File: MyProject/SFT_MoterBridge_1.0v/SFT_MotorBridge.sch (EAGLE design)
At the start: 44 parts

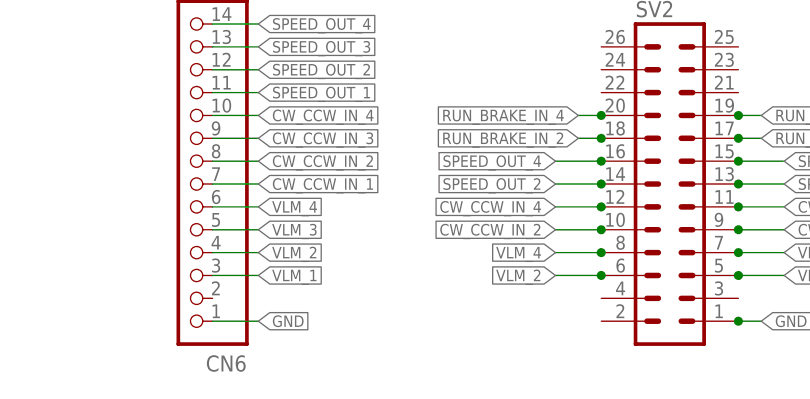
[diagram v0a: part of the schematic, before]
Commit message: kyuukei reset
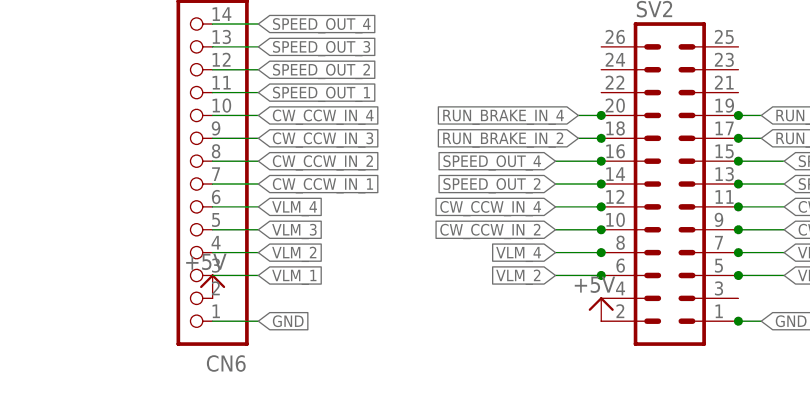
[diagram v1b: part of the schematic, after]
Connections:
- net +5V: now also CN6.2, SV2.2
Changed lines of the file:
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@@
 <part name="R23" library="01_R" deviceset="RESISTOR__SMD" device=""/>
 <part name="R24" library="01_R" deviceset="RESISTOR__SMD" device=""/>
+<part name="U$26" library="09_OTHER" deviceset="+5V" device=""/>
+<part name="U$35" library="09_OTHER" deviceset="+5V" device=""/>
 </parts>
 <sheets>
@@
 <instance part="R23" gate="G$1" x="63.5" y="10.16" rot="R90"/>
 <instance part="R24" gate="G$1" x="91.44" y="10.16" rot="R90"/>
+<instance part="U$26" gate="G$1" x="154.94" y="12.7"/>
+<instance part="U$35" gate="G$1" x="198.12" y="10.16"/>
 </instances>
 <busses>
@@
 <pinref part="R24" gate="G$1" pin="P$2"/>
 </segment>
-</net>
+<segment>
+<pinref part="CN6" gate="G$1" pin="2"/>
+<pinref part="U$26" gate="G$1" pin="+5V"/>
+</segment>
+<segment>
+<pinref part="SV2" gate="1" pin="2"/>
+<pinref part="U$35" gate="G$1" pin="+5V"/>
+</segment>
+</net>

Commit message: test2
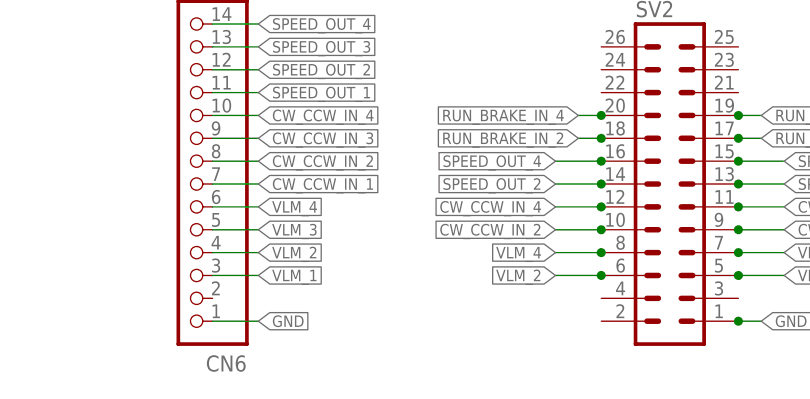
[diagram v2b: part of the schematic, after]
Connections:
- net +5V: no longer CN6.2, SV2.2
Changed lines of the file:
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@@
 <part name="R23" library="01_R" deviceset="RESISTOR__SMD" device=""/>
 <part name="R24" library="01_R" deviceset="RESISTOR__SMD" device=""/>
-<part name="U$26" library="09_OTHER" deviceset="+5V" device=""/>
-<part name="U$35" library="09_OTHER" deviceset="+5V" device=""/>
 </parts>
 <sheets>
@@
 <instance part="R23" gate="G$1" x="63.5" y="10.16" rot="R90"/>
 <instance part="R24" gate="G$1" x="91.44" y="10.16" rot="R90"/>
-<instance part="U$26" gate="G$1" x="154.94" y="12.7"/>
-<instance part="U$35" gate="G$1" x="198.12" y="10.16"/>
 </instances>
 <busses>
@@
 <pinref part="R24" gate="G$1" pin="P$2"/>
 </segment>
-<segment>
-<pinref part="CN6" gate="G$1" pin="2"/>
-<pinref part="U$26" gate="G$1" pin="+5V"/>
-</segment>
-<segment>
-<pinref part="SV2" gate="1" pin="2"/>
-<pinref part="U$35" gate="G$1" pin="+5V"/>
-</segment>
-</net>
+</net>
